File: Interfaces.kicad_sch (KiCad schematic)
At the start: 11 parts, among them J1 I/O_HDR, J24 SWDB, J4 I2C1_Headers, J5 UART1_HDR

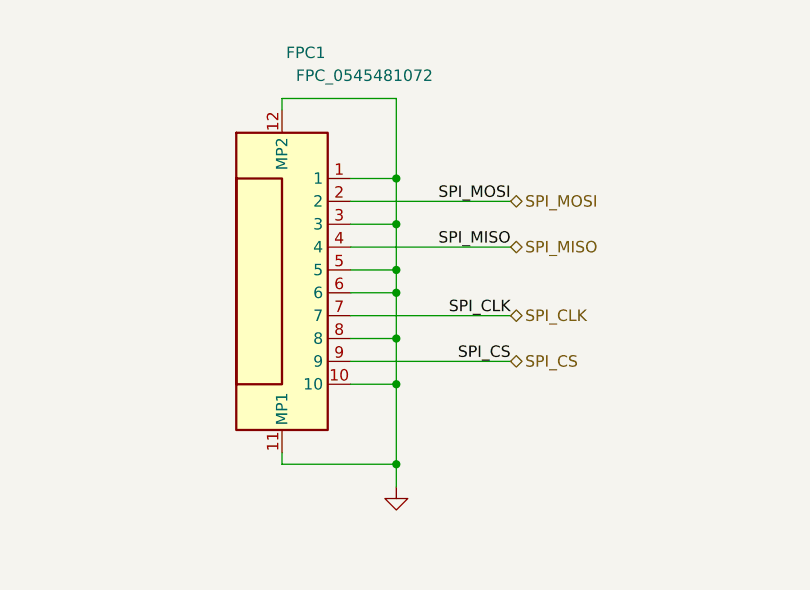
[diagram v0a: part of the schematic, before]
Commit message: Update
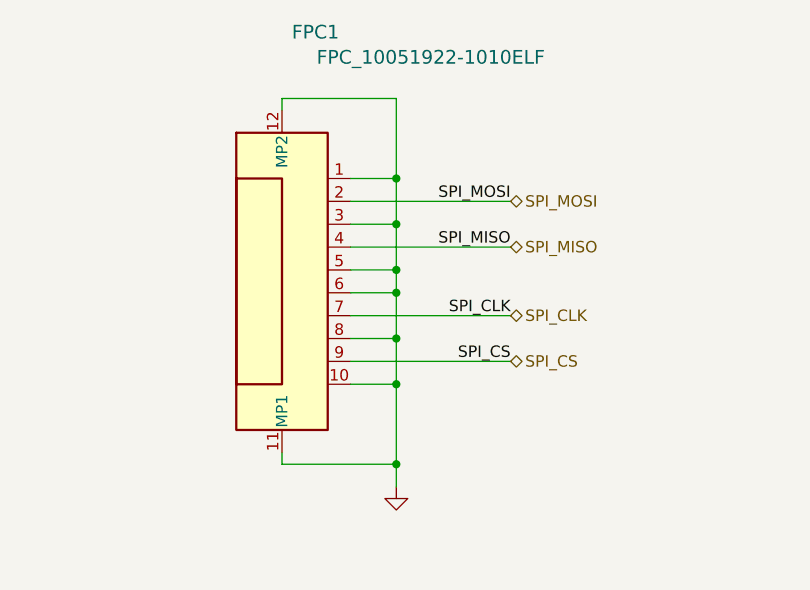
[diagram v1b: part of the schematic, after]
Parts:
- removed FPC1: FPC_0545481072, Personal_Project:FPC_0545481072, symbol Personal_Projects:FPC_0545481072
- added FPC1: FPC_10051922-1010ELF, Personal_Project:FPC_10051922_1010, symbol Personal_Projects:FPC_10051922-1010ELF
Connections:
- net GND: now also FPC1.1, FPC1.10, FPC1.11 (MP1), FPC1.12 (MP2), FPC1.3, FPC1.5, FPC1.6, FPC1.8
- net SPI_CLK: now also FPC1.7
- net SPI_CS: now also FPC1.9
- net SPI_MISO: now also FPC1.4
- net SPI_MOSI: now also FPC1.2
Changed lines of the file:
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@@
-	)
-	(symbol
-		(lib_id "Personal_Projects:FPC_0545481072")
-		(at 53.34 41.91 0)
-		(unit 1)
-		(exclude_from_sim no)
-		(in_bom yes)
-		(on_board yes)
-		(dnp no)
-		(property "Reference" "FPC1"
-			(at 63.246 27.94 0)
-			(effects
-				(font
-					(size 1.27 1.27)
-				)
-				(justify right)
-			)
-		)
-		(property "Value" "FPC_0545481072"
-			(at 75.184 30.48 0)
-			(effects
-				(font
-					(size 1.27 1.27)
-				)
-				(justify right)
-			)
-		)
-		(property "Footprint" "Personal_Project:FPC_0545481072"
-			(at 74.93 136.83 0)
-			(effects
-				(font
-					(size 1.27 1.27)
-				)
-				(justify left top)
-				(hide yes)
-			)
-		)
-		(property "Datasheet" "https://www.molex.com/en-us/products/part-detail-pdf/545481072?display=pdf"
-			(at 74.93 236.83 0)
-			(effects
-				(font
-					(size 1.27 1.27)
-				)
-				(justify left top)
-				(hide yes)
-			)
-		)
-		(property "Description" "0.50mm Pitch Easy-On FFC/FPC Connector, 1.20mm Height, Right-Angle, Surface Mount, ZIF, Bottom Contact Style, 10 Circuits, Gold (Au) Plating"
-			(at 53.34 72.39 0)
-			(effects
-				(font
-					(size 1.27 1.27)
-				)
-				(hide yes)
-			)
-		)
-		(property "Height" "1.3"
-			(at 74.93 436.83 0)
-			(effects
-				(font
-					(size 1.27 1.27)
-				)
-				(justify left top)
-				(hide yes)
-			)
-		)
-		(property "Arrow Part Number" "0545481072"
-			(at 74.93 536.83 0)
-			(effects
-				(font
-					(size 1.27 1.27)
-				)
-				(justify left top)
-				(hide yes)
-			)
-		)
-		(property "Arrow Price/Stock" ""
-			(at 74.93 636.83 0)
-			(effects
-				(font
-					(size 1.27 1.27)
-				)
-				(justify left top)
-				(hide yes)
-			)
-		)
-		(property "Manufacturer_Name" "Molex"
-			(at 74.93 736.83 0)
-			(effects
-				(font
-					(size 1.27 1.27)
-				)
-				(justify left top)
-				(hide yes)
-			)
-		)
-		(property "Manufacturer_Part_Number" "0545481072"
-			(at 74.93 836.83 0)
-			(effects
-				(font
-					(size 1.27 1.27)
-				)
-				(justify left top)
-				(hide yes)
-			)
-		)
-		(pin "4"
-		)
-		(pin "7"
-		)
-		(pin "6"
-		)
-		(pin "5"
-		)
-		(pin "2"
-		)
-		(pin "8"
-		)
-		(pin "3"
-		)
-		(pin "10"
-		)
-		(pin "12"
-		)
-		(pin "11"
-		)
-		(pin "9"
-		)
-		(pin "1"
-		)
-		(instances
-			(project "Bluetooth_Board"
-				(path "/05989bb3-969e-4aaa-b344-5f0e2d5af968/abc98c8d-e19e-4e25-aa44-7b8f1ef72b8d"
-					(reference "FPC1")
-					(unit 1)
-				)
-			)
-		)
 	)
 	(symbol
@@
 					(unit 1)
 				)
+			)
+		)
+	)
+	(symbol
+		(lib_id "Personal_Projects:FPC_10051922-1010ELF")
+		(at 53.34 41.91 0)
+		(unit 1)
+		(exclude_from_sim no)
+		(in_bom yes)
+		(on_board yes)
+		(dnp no)
+		(property "Reference" "FPC1"
+			(at 64.77 25.654 0)
+			(effects
+				(font
+					(size 1.524 1.524)
+				)
+				(justify right)
+			)
+		)
+		(property "Value" "FPC_10051922-1010ELF"
+			(at 87.63 28.448 0)
+			(effects
+				(font
+					(size 1.524 1.524)
+				)
+				(justify right)
+			)
+		)
+		(property "Footprint" "Personal_Project:FPC_10051922_1010"
+			(at 53.34 88.9 0)
+			(effects
+				(font
+					(size 1.27 1.27)
+					(italic yes)
+				)
+				(hide yes)
+			)
+		)
+		(property "Datasheet" "10051922-1010ELF"
+			(at 53.34 85.09 0)
+			(effects
+				(font
+					(size 1.27 1.27)
+					(italic yes)
+				)
+				(hide yes)
+			)
+		)
+		(property "Description" ""
+			(at 66.04 41.91 0)
+			(effects
+				(font
+					(size 1.27 1.27)
+				)
+				(hide yes)
+			)
+		)
+		(pin "6"
+		)
+		(pin "9"
+		)
+		(pin "4"
+		)
+		(pin "7"
+		)
+		(pin "2"
+		)
+		(pin "5"
+		)
+		(pin "3"
+		)
+		(pin "8"
+		)
+		(pin "12"
+		)
+		(pin "10"
+		)
+		(pin "1"
+		)
+		(pin "11"
+		)
+		(instances
+			(project "Bluetooth_Board"
+				(path "/05989bb3-969e-4aaa-b344-5f0e2d5af968/abc98c8d-e19e-4e25-aa44-7b8f1ef72b8d"
+					(reference "FPC1")
+					(unit 1)
+				)
